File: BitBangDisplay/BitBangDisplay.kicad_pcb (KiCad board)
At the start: 2 copper layers, 100 x 88 mm, 78 parts, among them J1 Conn_01x04, J10 Conn_01x20, J11 Conn_01x01, J12 Conn_01x01, J13 KeyerJack, J14 KeyerJack, J15 KeyerJack, J16 SPEAKER, J2 Audio-Jack-3_2Switches, J20 Conn_01x01, J21 Conn_01x01, J3 Conn_01x01, J4 Conn_01x01, J5 Conn_01x01, J6 Conn_01x01, J7 Conn_01x01, J8 Conn_01x01, J9 Conn_01x01, SW1 SW_Push, SW2 SW_Push, SW3 SW_Push, SW4 SW_Push, SW5 SW_Push, U1 LCD1602ExtraPins, U2 LM358, U5 LCD1602ExtraPins

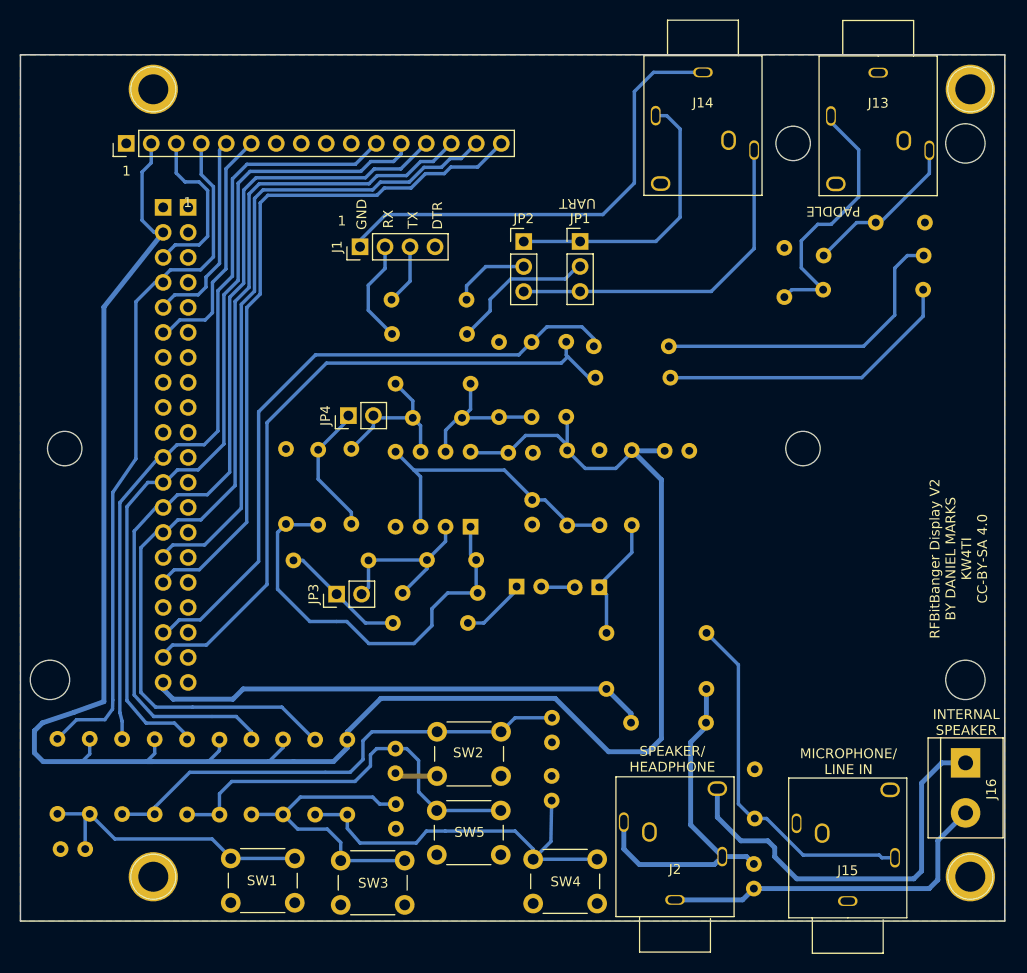
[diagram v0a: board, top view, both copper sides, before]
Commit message: Converted all Kicad projects to version 6.0.10
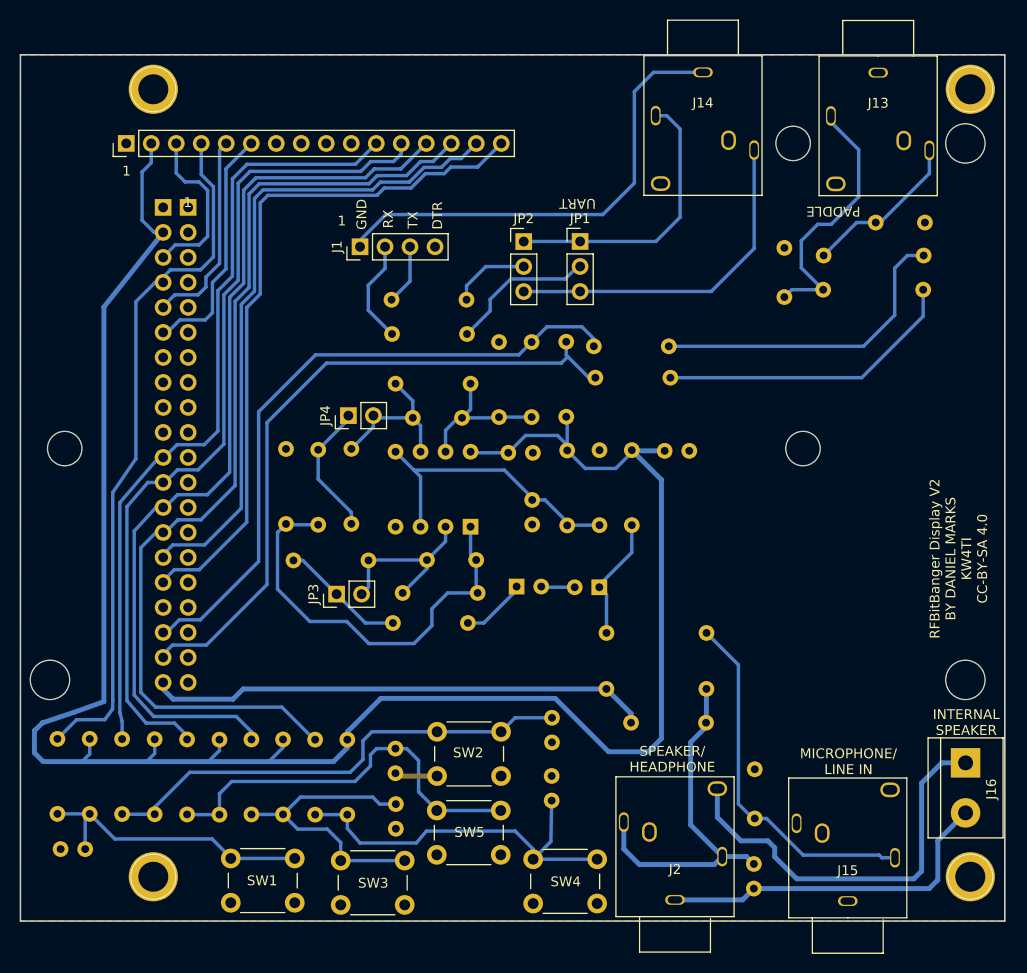
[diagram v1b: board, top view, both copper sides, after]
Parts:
- C12, C9: value 1 nF -> 100 pF
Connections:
- C8 pad 2: Net-(C8-Pad2) -> +5V
- J1 pad 4: (no net) -> unconnected-(J1-Pad4)
- J15 pad 2: (no net) -> unconnected-(J15-Pad2)
- J2 pad 5: (no net) -> unconnected-(J2-Pad5)
- R11 pad 2: Net-(C8-Pad2) -> +5V
- R14 pad 1: Net-(C8-Pad2) -> +5V
- U1 pad 10: (no net) -> unconnected-(U1-Pad10)
- U1 pad 7: (no net) -> unconnected-(U1-Pad7)
- U1 pad 8: (no net) -> unconnected-(U1-Pad8)
- U1 pad 9: (no net) -> unconnected-(U1-Pad9)
- U2 pad 3: Net-(C8-Pad2) -> +5V
- U2 pad 5: Net-(C8-Pad2) -> +5V
- U5 pad 10: (no net) -> unconnected-(U5-Pad10)
- U5 pad 7: (no net) -> unconnected-(U5-Pad7)
- U5 pad 8: (no net) -> unconnected-(U5-Pad8)
- U5 pad 9: (no net) -> unconnected-(U5-Pad9)
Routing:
- net Net-(C8-Pad2): track 30.2 -> 0.00 mm
- net +5V: track 212.0 -> 242.1 mm
- net Net-(C11-Pad2): track 42.9 -> 41.1 mm
- net DB4: track 81.2 -> 80.3 mm
- net Net-(R46-Pad1): track 40.5 -> 39.8 mm
- net Net-(C9-Pad1): track 18.9 -> 18.2 mm
- net Net-(JP2-Pad1): track 29.5 -> 28.9 mm
- net RW: track 21.3 -> 20.7 mm
- net DB7: track 100.5 -> 99.9 mm
- net GND: track 40.4 -> 39.9 mm
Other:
- net class Default removed
